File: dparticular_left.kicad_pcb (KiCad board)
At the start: 2 copper layers, 51 parts, among them J1 To Left Hand, SW1:10 Key_Ins, SW1:11 Key_Prnt, SW2:10 Key_F7, SW2:11 Key_F8, SW2:12 Key_F9, SW2:13 Key_F10, SW2:14 Key_F11, SW2:15 Key_F12, SW2:16 Key_Del, SW3:10 Key_7, SW3:11 Key_8, SW3:12 Key_9, SW3:13 Key_0, SW3:14 Key_Hyph, SW3:15 Key_Eql, SW3:16 Key_Bksp, SW3:9 Key_6, SW4:10 Key_U, SW4:11 Key_I, SW4:12 Key_O, SW4:13 Key_P, SW4:14 Key_LBrk, SW4:15 Key_RBrk, SW4:16 Key_BkSl, SW4:9 Key_Y, SW5:10 Key_J, SW5:11 Key_K, SW5:12 Key_L, SW5:13 Key_Semi, SW5:14 Key_Quot, SW5:16 Key_Entr, SW5:9 Key_H, SW6:10 Key_M, SW6:11 Key_Coma, SW6:12 Key_Per, SW6:13 Key_Slsh, SW6:14 Key_RShft, SW6:9 Key_N, SW7:11 Key_RAlt, SW7:12 Key_RWin, SW7:13 Key_Menu, SW7:14 Key_RCtrl, SW7:9 Key_RSpc, U1 MCP23018

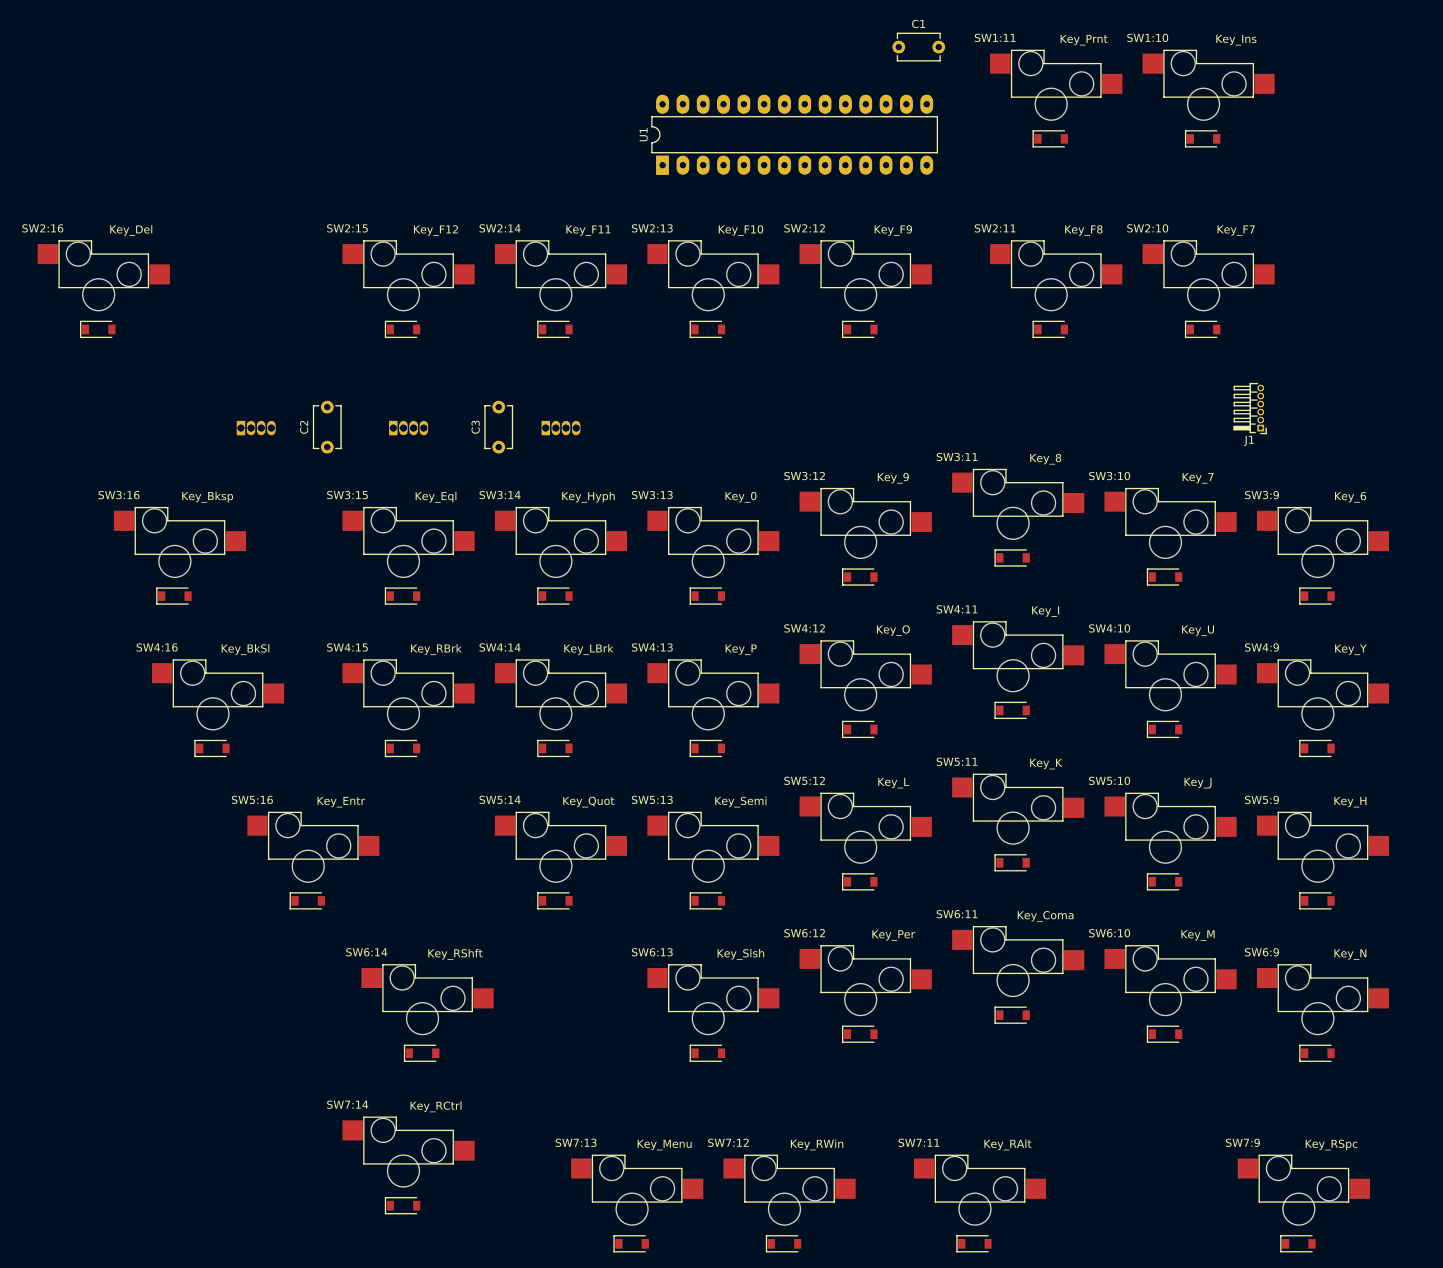
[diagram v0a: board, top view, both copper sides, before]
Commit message: Preliminary placements for left hand
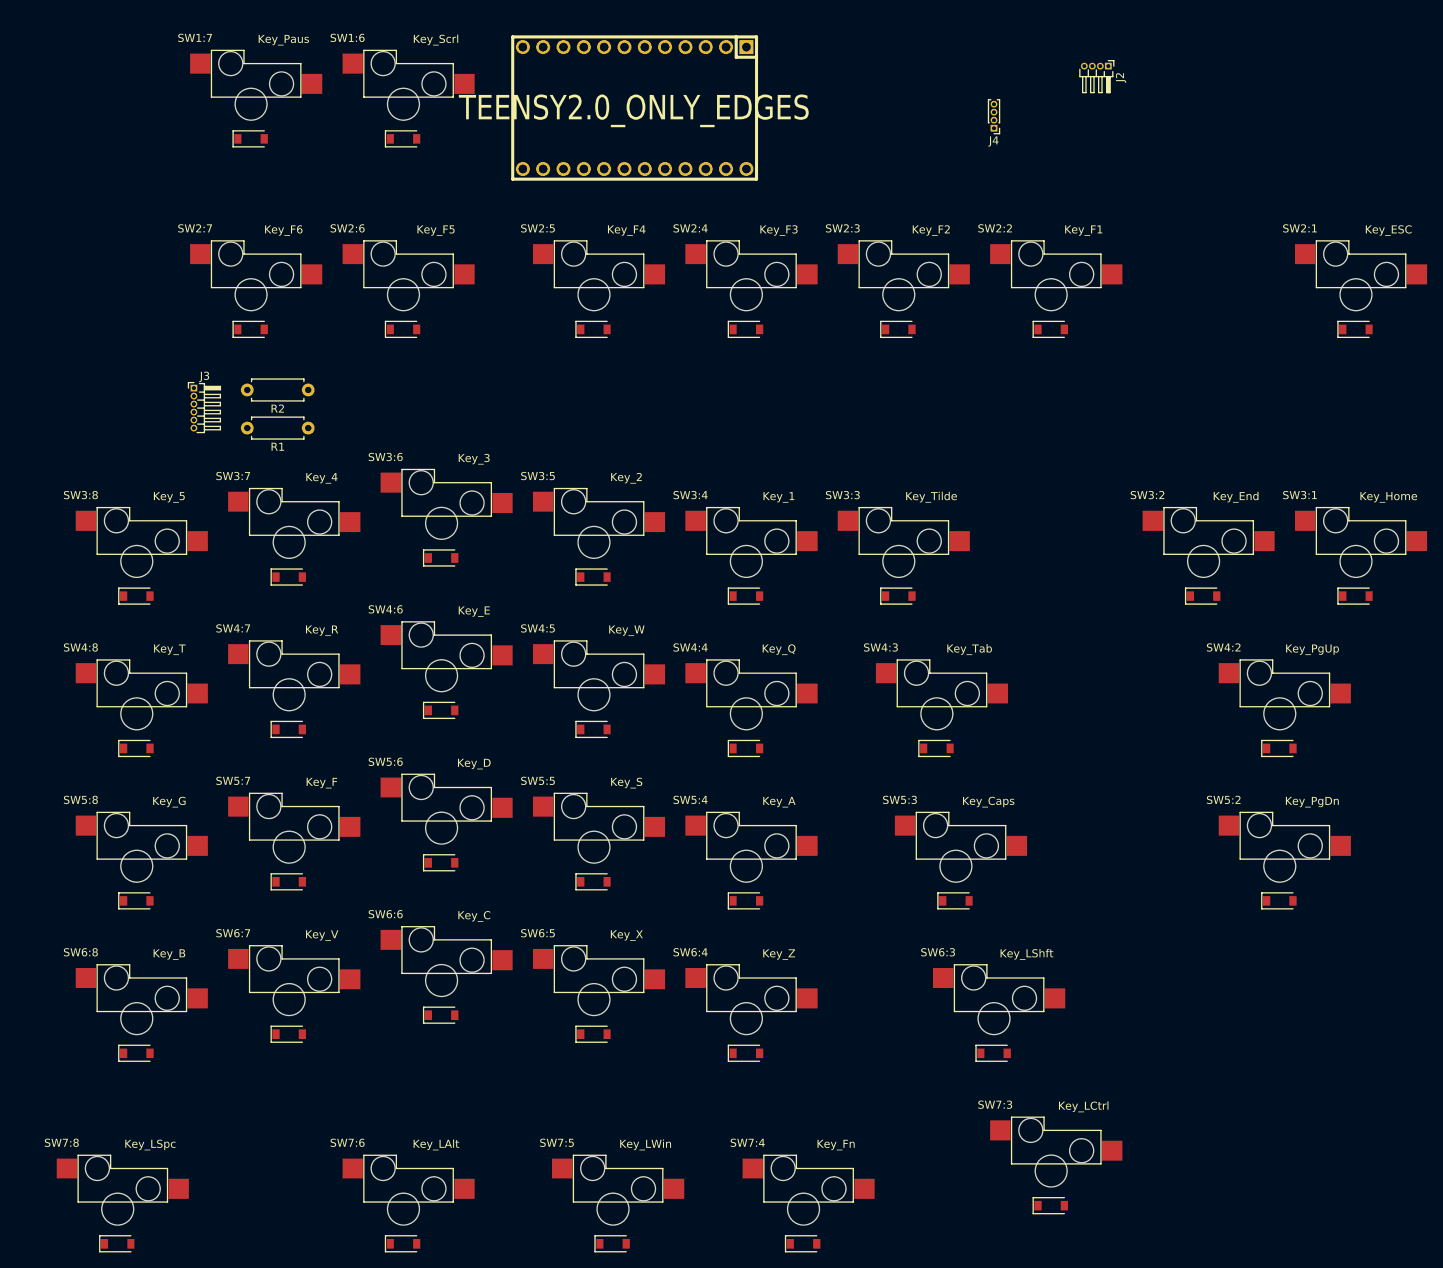
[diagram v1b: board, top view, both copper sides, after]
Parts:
- removed C1, C2, C3: 0.1uF, Capacitor_THT:C_Disc_D5.1mm_W3.2mm_P5.00mm
- removed D1, D2, D3: APA-106-F5, LED_THT:LED_D5.0mm-4_RGB
- removed J1: To Left Hand, Connector_PinHeader_1.00mm:PinHeader_1x06_P1.00mm_Horizontal
- removed SW1:10: Key_Ins, dparticular:MX_W_DIODE
- removed SW1:11: Key_Prnt, dparticular:MX_W_DIODE
- removed SW2:10: Key_F7, dparticular:MX_W_DIODE
- removed SW2:11: Key_F8, dparticular:MX_W_DIODE
- removed SW2:12: Key_F9, dparticular:MX_W_DIODE
- removed SW2:13: Key_F10, dparticular:MX_W_DIODE
- removed SW2:14: Key_F11, dparticular:MX_W_DIODE
- removed SW2:15: Key_F12, dparticular:MX_W_DIODE
- removed SW2:16: Key_Del, dparticular:MX_W_DIODE
- removed SW3:10: Key_7, dparticular:MX_W_DIODE
- removed SW3:11: Key_8, dparticular:MX_W_DIODE
- removed SW3:12: Key_9, dparticular:MX_W_DIODE
- removed SW3:13: Key_0, dparticular:MX_W_DIODE
- removed SW3:14: Key_Hyph, dparticular:MX_W_DIODE
- removed SW3:15: Key_Eql, dparticular:MX_W_DIODE
- removed SW3:16: Key_Bksp, dparticular:MX_W_DIODE
- removed SW3:9: Key_6, dparticular:MX_W_DIODE
- removed SW4:10: Key_U, dparticular:MX_W_DIODE
- removed SW4:11: Key_I, dparticular:MX_W_DIODE
- removed SW4:12: Key_O, dparticular:MX_W_DIODE
- removed SW4:13: Key_P, dparticular:MX_W_DIODE
- removed SW4:14: Key_LBrk, dparticular:MX_W_DIODE
- removed SW4:15: Key_RBrk, dparticular:MX_W_DIODE
- removed SW4:16: Key_BkSl, dparticular:MX_W_DIODE
- removed SW4:9: Key_Y, dparticular:MX_W_DIODE
- removed SW5:10: Key_J, dparticular:MX_W_DIODE
- removed SW5:11: Key_K, dparticular:MX_W_DIODE
- removed SW5:12: Key_L, dparticular:MX_W_DIODE
- removed SW5:13: Key_Semi, dparticular:MX_W_DIODE
- removed SW5:14: Key_Quot, dparticular:MX_W_DIODE
- removed SW5:16: Key_Entr, dparticular:MX_W_DIODE
- removed SW5:9: Key_H, dparticular:MX_W_DIODE
- removed SW6:10: Key_M, dparticular:MX_W_DIODE
- removed SW6:11: Key_Coma, dparticular:MX_W_DIODE
- removed SW6:12: Key_Per, dparticular:MX_W_DIODE
- removed SW6:13: Key_Slsh, dparticular:MX_W_DIODE
- removed SW6:14: Key_RShft, dparticular:MX_W_DIODE
- removed SW6:9: Key_N, dparticular:MX_W_DIODE
- removed SW7:11: Key_RAlt, dparticular:MX_W_DIODE
- removed SW7:12: Key_RWin, dparticular:MX_W_DIODE
- removed SW7:13: Key_Menu, dparticular:MX_W_DIODE
- removed SW7:14: Key_RCtrl, dparticular:MX_W_DIODE
- removed SW7:9: Key_RSpc, dparticular:MX_W_DIODE
- removed U1: MCP23018, Package_DIP:DIP-28_W7.62mm_LongPads
- added J2: USB from outside, Connector_PinHeader_1.00mm:PinHeader_1x04_P1.00mm_Horizontal, F.Cu at (164.3, 28.6)
- added J3: To Right Hand, Connector_PinHeader_1.00mm:PinHeader_1x06_P1.00mm_Horizontal, F.Cu at (50.0, 68.8)
- added J4: Jumper to Teensy USB, Connector_PinHeader_1.00mm:PinHeader_1x04_P1.00mm_Vertical, F.Cu at (150.0, 36.3)
- added R1: 4.7k, Resistor_THT:R_Axial_DIN0207_L6.3mm_D2.5mm_P7.62mm_Horizontal, F.Cu at (64.3, 73.8)
- added R2: 4.7k, Resistor_THT:R_Axial_DIN0207_L6.3mm_D2.5mm_P7.62mm_Horizontal, F.Cu at (64.3, 69.1)
- added SW1:6: Key_Scrl, dparticular:MX_W_DIODE, F.Cu at (76.2, 33.3)
- added SW1:7: Key_Paus, dparticular:MX_W_DIODE, F.Cu at (57.1, 33.3)
- added SW2:1: Key_ESC, dparticular:MX_W_DIODE, F.Cu at (195.3, 57.1)
- added SW2:2: Key_F1, dparticular:MX_W_DIODE, F.Cu at (157.2, 57.1)
- added SW2:3: Key_F2, dparticular:MX_W_DIODE, F.Cu at (138.1, 57.1)
- added SW2:4: Key_F3, dparticular:MX_W_DIODE, F.Cu at (119.1, 57.1)
- added SW2:5: Key_F4, dparticular:MX_W_DIODE, F.Cu at (100.0, 57.1)
- added SW2:6: Key_F5, dparticular:MX_W_DIODE, F.Cu at (76.2, 57.1)
- added SW2:7: Key_F6, dparticular:MX_W_DIODE, F.Cu at (57.1, 57.1)
- added SW3:1: Key_Home, dparticular:MX_W_DIODE, F.Cu at (195.3, 90.5)
- added SW3:2: Key_End, dparticular:MX_W_DIODE, F.Cu at (176.2, 90.5)
- added SW3:3: Key_Tilde, dparticular:MX_W_DIODE, F.Cu at (138.1, 90.5)
- added SW3:4: Key_1, dparticular:MX_W_DIODE, F.Cu at (119.1, 90.5)
- added SW3:5: Key_2, dparticular:MX_W_DIODE, F.Cu at (100.0, 88.1)
- added SW3:6: Key_3, dparticular:MX_W_DIODE, F.Cu at (81.0, 85.7)
- added SW3:7: Key_4, dparticular:MX_W_DIODE, F.Cu at (61.9, 88.1)
- added SW3:8: Key_5, dparticular:MX_W_DIODE, F.Cu at (42.9, 90.5)
- added SW4:2: Key_PgUp, dparticular:MX_W_DIODE, F.Cu at (185.7, 109.5)
- added SW4:3: Key_Tab, dparticular:MX_W_DIODE, F.Cu at (142.9, 109.5)
- added SW4:4: Key_Q, dparticular:MX_W_DIODE, F.Cu at (119.1, 109.5)
- added SW4:5: Key_W, dparticular:MX_W_DIODE, F.Cu at (100.0, 107.2)
- added SW4:6: Key_E, dparticular:MX_W_DIODE, F.Cu at (81.0, 104.8)
- added SW4:7: Key_R, dparticular:MX_W_DIODE, F.Cu at (61.9, 107.2)
- added SW4:8: Key_T, dparticular:MX_W_DIODE, F.Cu at (42.9, 109.5)
- added SW5:2: Key_PgDn, dparticular:MX_W_DIODE, F.Cu at (185.7, 128.6)
- added SW5:3: Key_Caps, dparticular:MX_W_DIODE, F.Cu at (145.3, 128.6)
- added SW5:4: Key_A, dparticular:MX_W_DIODE, F.Cu at (119.1, 128.6)
- added SW5:5: Key_S, dparticular:MX_W_DIODE, F.Cu at (100.0, 126.2)
- added SW5:6: Key_D, dparticular:MX_W_DIODE, F.Cu at (81.0, 123.8)
- added SW5:7: Key_F, dparticular:MX_W_DIODE, F.Cu at (61.9, 126.2)
- added SW5:8: Key_G, dparticular:MX_W_DIODE, F.Cu at (42.9, 128.6)
- added SW6:3: Key_LShft, dparticular:MX_W_DIODE, F.Cu at (150.0, 147.6)
- added SW6:4: Key_Z, dparticular:MX_W_DIODE, F.Cu at (119.1, 147.6)
- added SW6:5: Key_X, dparticular:MX_W_DIODE, F.Cu at (100.0, 145.3)
- added SW6:6: Key_C, dparticular:MX_W_DIODE, F.Cu at (81.0, 142.9)
- added SW6:7: Key_V, dparticular:MX_W_DIODE, F.Cu at (61.9, 145.3)
- added SW6:8: Key_B, dparticular:MX_W_DIODE, F.Cu at (42.9, 147.6)
- added SW7:3: Key_LCtrl, dparticular:MX_W_DIODE, F.Cu at (157.2, 166.7)
- added SW7:4: Key_Fn, dparticular:MX_W_DIODE, F.Cu at (126.2, 171.4)
- added SW7:5: Key_LWin, dparticular:MX_W_DIODE, F.Cu at (102.4, 171.4)
- added SW7:6: Key_LAlt, dparticular:MX_W_DIODE, F.Cu at (76.2, 171.4)
- added SW7:8: Key_LSpc, dparticular:MX_W_DIODE, F.Cu at (40.5, 171.4)
- added U2: TEENSY2.0_ONLY_EDGES, dparticular:TEENSY_2.0_EDGES_ONLY, F.Cu at (105.1, 33.8)
